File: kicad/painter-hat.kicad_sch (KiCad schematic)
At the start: 27 parts, among them J1 Conn_01x08_Socket, J2 Conn_01x08_Socket, J3 Conn_01x08_Socket, J4 Conn_01x08_Socket, J5 Conn_02x20_Odd_Even, J6 Conn_01x04, J9 Conn_01x04, Q1 NPN, Q2 NPN, U1 MAX26405AFOAY+T, Y2 16 MHz

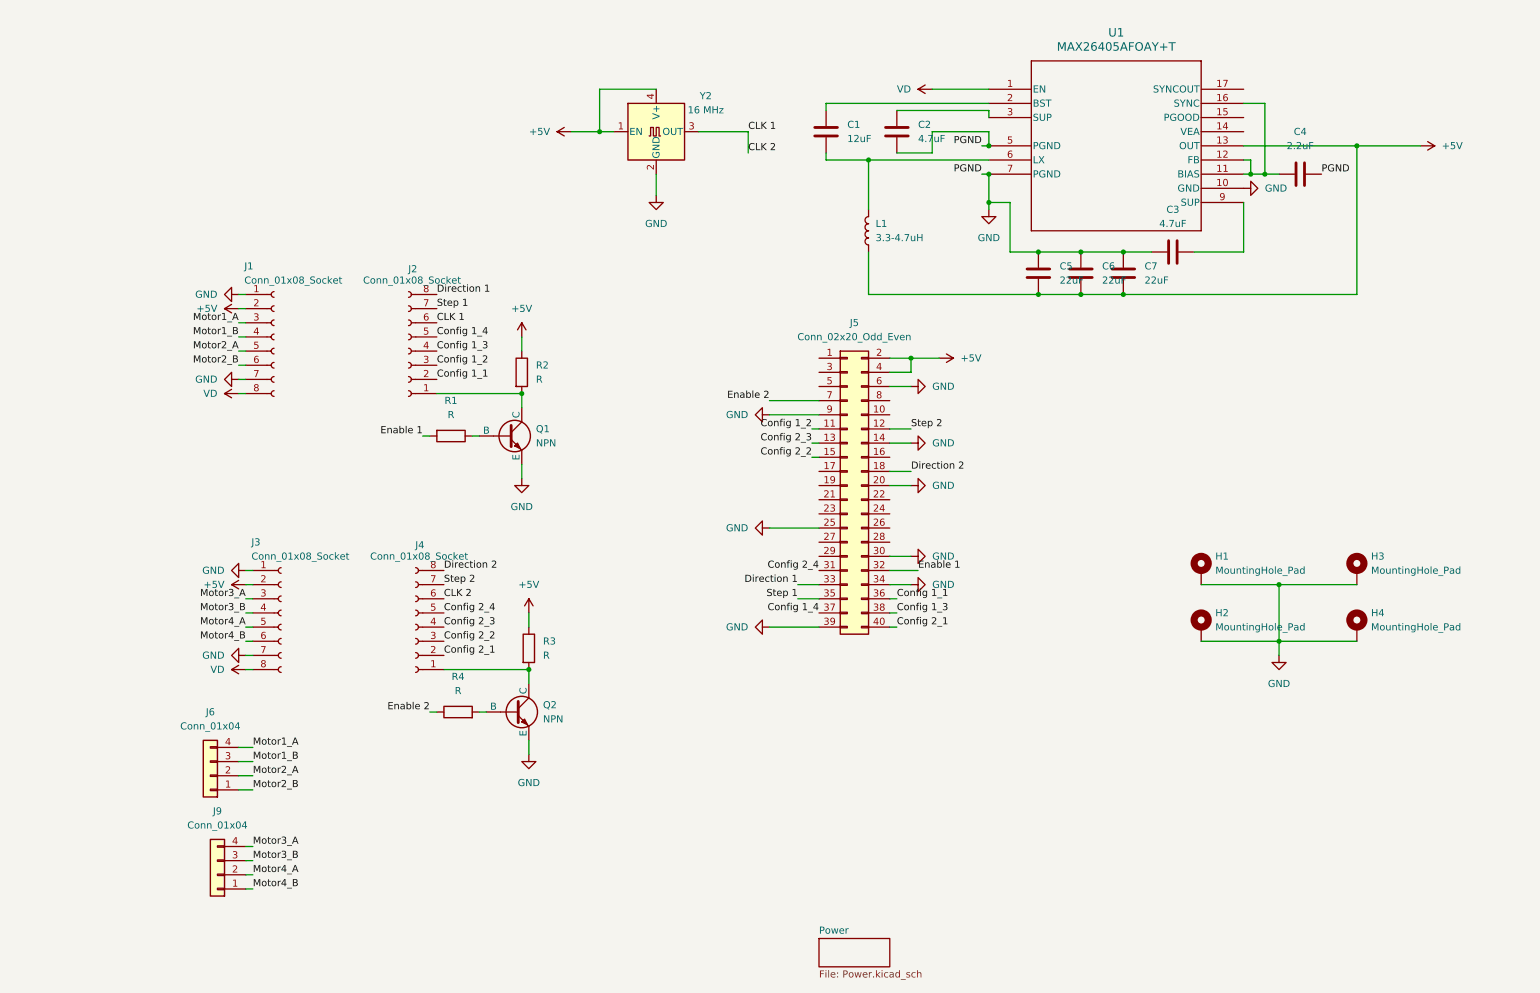
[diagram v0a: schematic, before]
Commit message: feat: v2
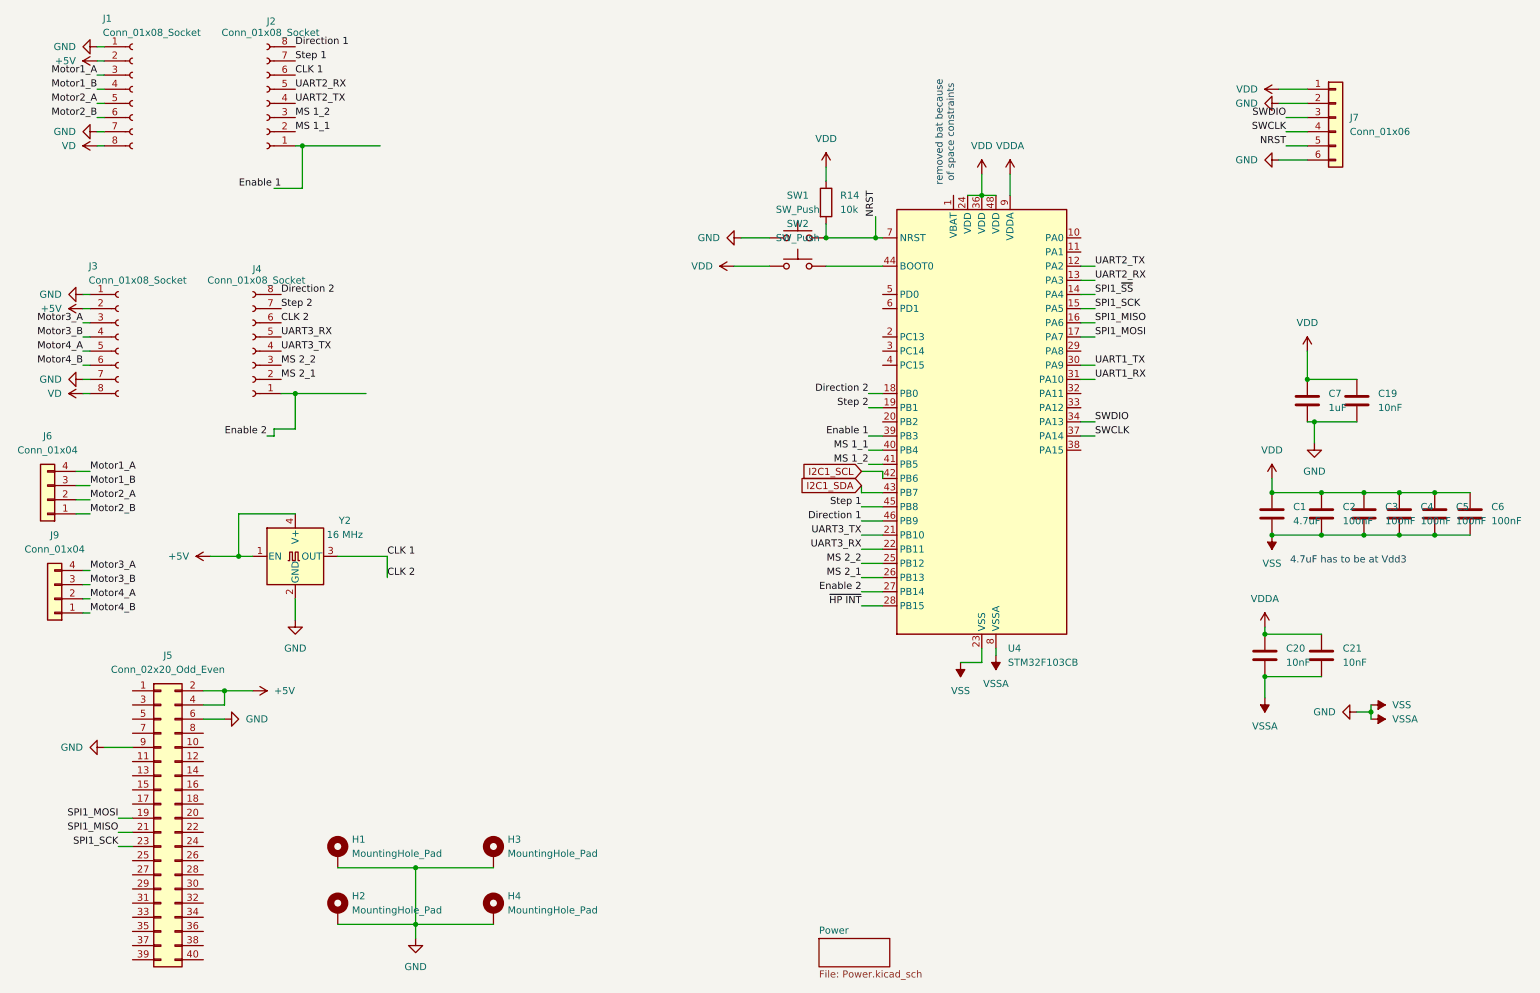
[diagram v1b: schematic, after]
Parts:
- removed L1: 3.3-4.7uH, Inductor_SMD:L_Coilcraft_XxL4030, symbol Device:L
- removed Q1, Q2: NPN, Package_TO_SOT_THT:TO-92L_Inline_Wide, symbol Simulation_SPICE:NPN
- removed R1, R2, R3, R4: R, Resistor_SMD:R_0603_1608Metric, symbol Device:R
- removed U1: MAX26405AFOAY+T, Own:FC2QFN-17, symbol Own:MAX26405AFOAY+T
- added C19, C20, C21: 10nF, Capacitor_SMD:C_0402_1005Metric, symbol Device:C
- added J7: Conn_01x06, Connector_PinSocket_2.54mm:PinSocket_1x06_P2.54mm_Vertical, symbol Connector_Generic:Conn_01x06
- added R14: 10k, Resistor_SMD:R_0402_1005Metric, symbol Device:R
- added SW1, SW2: SW_Push, Button_Switch_SMD:SW_Push_1P1T_NO_CK_KMR2, symbol Switch:SW_Push
- added U4: STM32F103CB, Package_QFP:LQFP-48_7x7mm_P0.5mm, symbol MCU_ST_STM32F1:STM32F103CBTx
- C1: value 12uF -> 4.7uF; footprint Capacitor_SMD:C_0603_1608Metric -> Capacitor_SMD:C_0402_1005Metric
- C2, C3: value 4.7uF -> 100nF; footprint Capacitor_SMD:C_0603_1608Metric -> Capacitor_SMD:C_0402_1005Metric
- C4: value 2.2uF -> 100nF; footprint Capacitor_SMD:C_0603_1608Metric -> Capacitor_SMD:C_0402_1005Metric
- C5, C6: value 22uF -> 100nF; footprint Capacitor_SMD:C_0805_2012Metric -> Capacitor_SMD:C_0402_1005Metric
- C7: value 22uF -> 1uF; footprint Capacitor_SMD:C_0805_2012Metric -> Capacitor_SMD:C_0603_1608Metric
- J1, J2, J3, J4: footprint Connector_PinHeader_2.54mm:PinHeader_1x08_P2.54mm_Vertical -> Connector_PinSocket_2.54mm:PinSocket_1x08_P2.54mm_Vertical
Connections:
- net +5V: no longer C5.2, C6.2, C7.2
- net Direction 1: now also U4.46 (PB9); no longer J5.33 (Pin_33)
- net Direction 2: now also U4.18 (PB0); no longer J5.18 (Pin_18)
- net Enable 1: now also J2.1 (Pin_1), U4.39 (PB3); no longer J5.32 (Pin_32)
- net Enable 2: now also J4.1 (Pin_1), U4.27 (PB14); no longer J5.7 (Pin_7)
- net GND: now also C1.2, C3.2, C5.2, C6.2, C7.2, C19.2, C20.2, C21.2, J7.2 (Pin_2), J7.6 (Pin_6), SW1.1, U4.23 (VSS), U4.35 (VSS), U4.47 (VSS), U4.8 (VSSA); no longer C3.1, C5.1, C6.1, C7.1, J5.14 (Pin_14), J5.20 (Pin_20), J5.25 (Pin_25), J5.30 (Pin_30), J5.34 (Pin_34), J5.39 (Pin_39)
- net Step 1: now also U4.45 (PB8); no longer J5.35 (Pin_35)
- net Step 2: now also U4.19 (PB1); no longer J5.12 (Pin_12)
- net SPI1_MOSI: now reaches J5.19 (Pin_19)
- net SPI1_MOSI: now also U4.17 (PA7)
- net SPI1_MISO: now reaches J5.21 (Pin_21)
- net SPI1_MISO: now also U4.16 (PA6)
- net SPI1_SCK: now reaches J5.23 (Pin_23)
- net SPI1_SCK: now also U4.15 (PA5)
- net VDD: now reaches C2.1
- net VDD: now also C1.1, C3.1, C4.1, C5.1, C6.1, C7.1, C19.1, J7.1 (Pin_1), R14.1, SW2.1, U4.24 (VDD), U4.36 (VDD), U4.48 (VDD)
- net Config 1_1: no longer names the net of J5.36 (Pin_36)
- net Config 1_1: no longer J2.2 (Pin_2)
- net Config 1_2: no longer names the net of J5.11 (Pin_11)
- net Config 1_2: no longer J2.3 (Pin_3)
- net Config 1_3: no longer names the net of J5.38 (Pin_38)
- net Config 1_3: no longer J2.4 (Pin_4)
- net Config 1_4: no longer names the net of J5.37 (Pin_37)
- net Config 1_4: no longer J2.5 (Pin_5)
- net Config 2_1: no longer names the net of J5.40 (Pin_40)
- net Config 2_1: no longer J4.2 (Pin_2)
- net Config 2_2: no longer names the net of J5.15 (Pin_15)
- net Config 2_2: no longer J4.3 (Pin_3)
- net Config 2_3: no longer names the net of J5.13 (Pin_13)
- net Config 2_3: no longer J4.4 (Pin_4)
- net Config 2_4: no longer names the net of J5.31 (Pin_31)
- net Config 2_4: no longer J4.5 (Pin_5)
- new net: SW2.2, U4.44 (BOOT0)
- new net I2C1_SCL: U4.42 (PB6)
- new net I2C1_SDA: U4.43 (PB7)
- new net MS 1_1: J2.2 (Pin_2), U4.40 (PB4)
- new net MS 1_2: J2.3 (Pin_3), U4.41 (PB5)
- new net MS 2_1: J4.2 (Pin_2), U4.26 (PB13)
- new net MS 2_2: J4.3 (Pin_3), U4.25 (PB12)
- new net NRST: J7.5 (Pin_5), R14.2, SW1.2, U4.7 (NRST)
- new net SPI1_~{SS}: U4.14 (PA4)
- new net SWCLK: J7.4 (Pin_4), U4.37 (PA14)
- new net SWDIO: J7.3 (Pin_3), U4.34 (PA13)
- new net UART1_RX: U4.31 (PA10)
- new net UART1_TX: U4.30 (PA9)
- new net UART2_RX: J2.5 (Pin_5), U4.13 (PA3)
- new net UART2_TX: J2.4 (Pin_4), U4.12 (PA2)
- new net UART3_RX: J4.5 (Pin_5), U4.22 (PB11)
- new net UART3_TX: J4.4 (Pin_4), U4.21 (PB10)
- new net VDDA: C20.1, C21.1, U4.9 (VDDA)
- new net ~{HP INT}: U4.28 (PB15)
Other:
- note added: "4.7uF has to be at Vdd3"
- note added: "removed bat because of space constraints"
- moved on the sheet: H1, H2, H3, H4, J1, J2, J3, J4, J5, J6, J9, Y2
